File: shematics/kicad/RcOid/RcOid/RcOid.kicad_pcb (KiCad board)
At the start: 2 copper layers, 30 x 26 mm, 7 parts, among them J1 Wemos Left (5V), J2 Wemos Right (3.3V), Q1 IRLX024N, U1 TSOP531xx

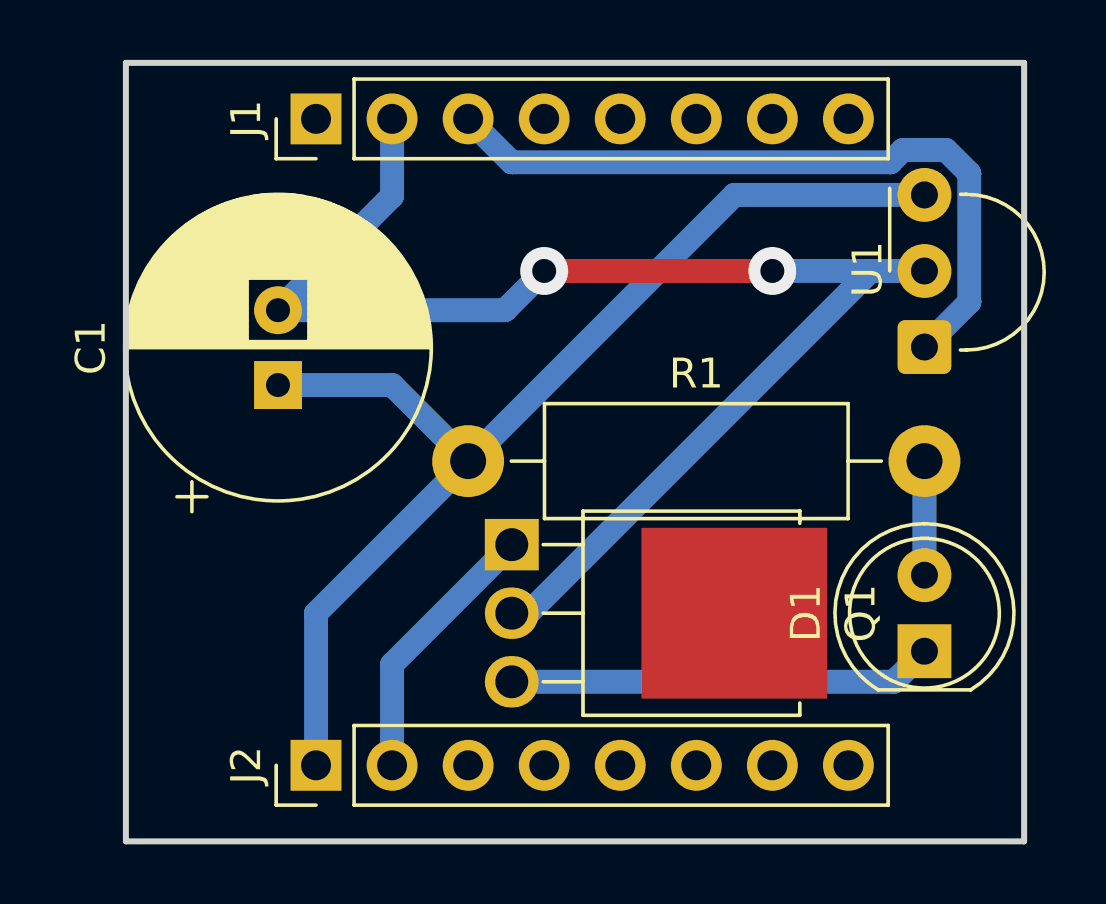
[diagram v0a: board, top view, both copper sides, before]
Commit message: TH PCB
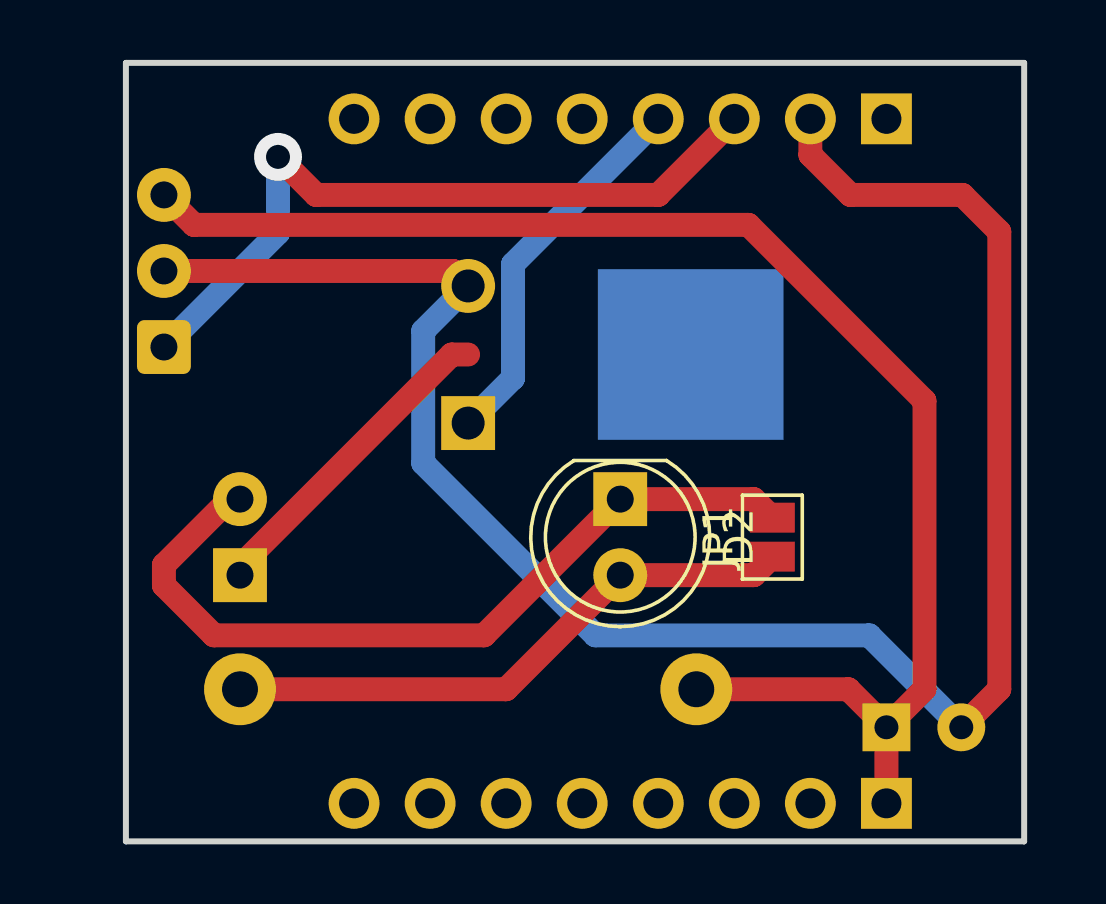
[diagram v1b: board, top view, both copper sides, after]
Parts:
- added D2: TRU 1577326, LED_THT:LED_D5.0mm_IRGrey, F.Cu at (139.7, 106.7)
- added JP1: SJ, Jumper:SolderJumper-2_P1.3mm_Open_Pad1.0x1.5mm, F.Cu at (144.8, 108.0)
- C1: value 3000µF -> 2000µF; moved to B.Cu
- D1: value LD271 -> TRU 1577326; footprint LED_THT:LED_D5.0mm_IRGrey -> LED_THT:LED_D5.0mm_Horizontal_O1.27mm_Z3.0mm_IRGrey; moved to B.Cu
- J1, J2, U1: moved to B.Cu
- Q1: value IRLX024N -> IRLU024N; footprint Package_TO_SOT_THT:TO-251-3-1EP_Horizontal_TabDown -> Package_TO_SOT_THT:TO-251-2-1EP_Horizontal_TabDown; moved to B.Cu
- R1: value 22 -> 47; moved to B.Cu
- moved U1 25.4 mm to (124.5, 101.6)
- moved C1 23.3 mm to (148.6, 114.3), turned to 0 degrees
- moved D1 23.0 mm to (127.0, 109.2)
- moved J2 19.1 mm to (148.6, 116.8)
- moved J1 19.1 mm to (148.6, 94.0)
- moved R1 10.8 mm to (142.2, 113.0), turned to 180 degrees
- moved Q1 4.31 mm to (134.6, 104.1), turned to 90 degrees
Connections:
- Q1 pad 1: Net-(J2-Pad2) -> Net-(J1-Pad4)
- Q1 pad 2: GND -> Net-(D1-Pad1)
- Q1 pad 3: Net-(D1-Pad1) -> GND
- R1 pad 2: Net-(D1-Pad2) -> Net-(D2-Pad2)
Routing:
- net Net-(D1-Pad2): track 3.81 -> 27.3 mm
- net Net-(D2-Pad2): track 0.00 -> 19.6 mm
- net GND: track 48.6 -> 64.2 mm, vias 2 -> 0
- net Net-(J1-Pad4): track 0.00 -> 12.8 mm
- net +3V3: track 38.6 -> 49.1 mm
- net Net-(J2-Pad2): track 9.03 -> 0.00 mm
- net Net-(D1-Pad1): track 14.2 -> 10.8 mm
- net Net-(J1-Pad3): track 24.3 -> 24.7 mm, vias 0 -> 1
